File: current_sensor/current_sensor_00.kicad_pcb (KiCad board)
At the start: 2 copper layers, 58.4 x 26.7 mm, 20 parts, among them J1 In, P1 Out, U1 MCP602

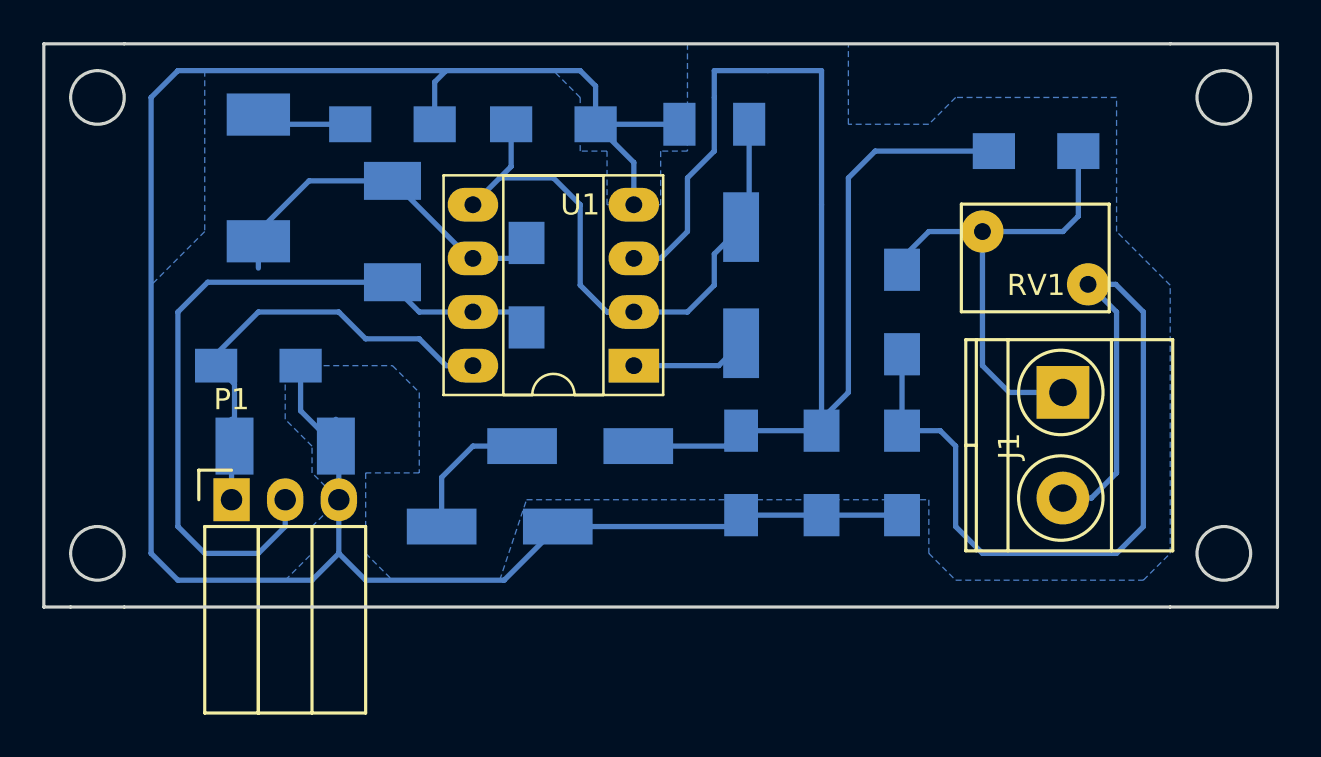
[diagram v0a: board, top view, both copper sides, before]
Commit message: template
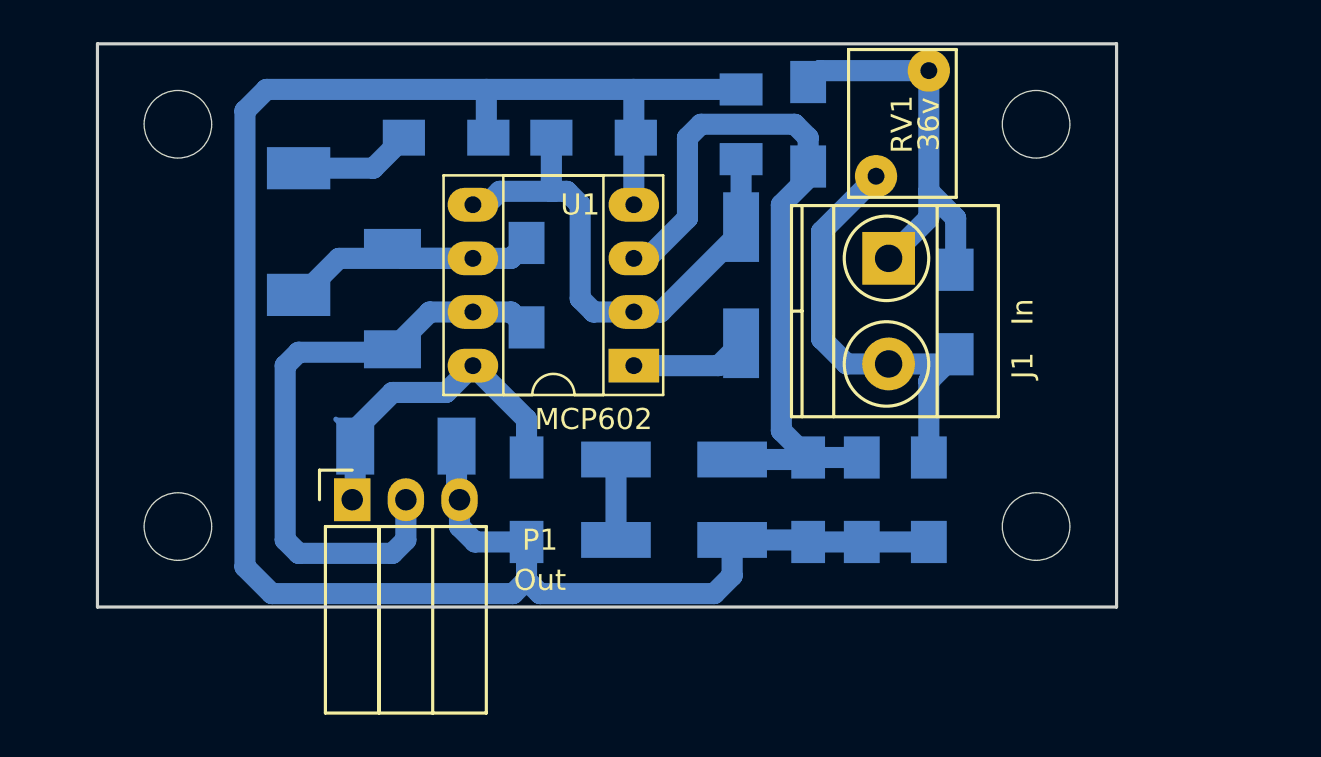
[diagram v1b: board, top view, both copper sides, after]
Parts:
- added ?: , Mounting_Holes:MountingHole_3.2mm_M3, F.Cu at (175.3, 114.3)
- added ?: , Mounting_Holes:MountingHole_3.2mm_M3, F.Cu at (175.3, 133.3)
- added ?: , Mounting_Holes:MountingHole_3.2mm_M3, F.Cu at (134.6, 133.3)
- added ?: , Mounting_Holes:MountingHole_3.2mm_M3, F.Cu at (134.6, 114.3)
- moved C5 14.2 mm to (151.1, 132.1), turned to 270 degrees
- moved R2 10.9 mm to (164.5, 114.3), turned to 270 degrees
- moved J1 10.4 mm to (168.3, 120.7)
- moved D2 8.28 mm to (158.1, 134.0)
- moved RV1 8.03 mm to (170.2, 111.8), turned to 270 degrees
- moved C4 5.72 mm to (145.4, 129.5)
- moved P1 5.72 mm to (142.9, 132.1)
- moved D1 4.49 mm to (158.1, 130.2)
- moved C3 3.42 mm to (164.5, 132.1)
- moved C8 3.18 mm to (144.8, 122.6)
- moved C7 3.17 mm to (140.3, 119.4)
- moved R8 2.62 mm to (147.3, 114.9)
- moved R1 2.54 mm to (171.4, 123.2)
- moved R5 2.29 mm to (167.0, 132.1)
- moved R7 2.01 mm to (154.3, 114.9)
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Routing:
- net Net-(C3-Pad1): track 63.7 -> 37.2 mm
- net /InB: track 46.1 -> 21.2 mm
- net GND: track 105.9 -> 98.0 mm
- net +5V: track 22.8 -> 15.8 mm
- net /Out: track 35.6 -> 30.2 mm
- net /InA: track 23.5 -> 19.9 mm
- net Net-(D1-Pad2): track 6.75 -> 3.81 mm
- net Net-(C6-Pad1): track 28.4 -> 26.1 mm
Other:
- board size 58.4 x 26.7 mm -> 48.3 x 26.7 mm
